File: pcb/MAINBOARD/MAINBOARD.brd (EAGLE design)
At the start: 85 x 56 mm, 67 parts, among them Q1 20MHz, SW1 P-DT6E, SW2 P-DT6E, T1 IRMLM0060TRPbF

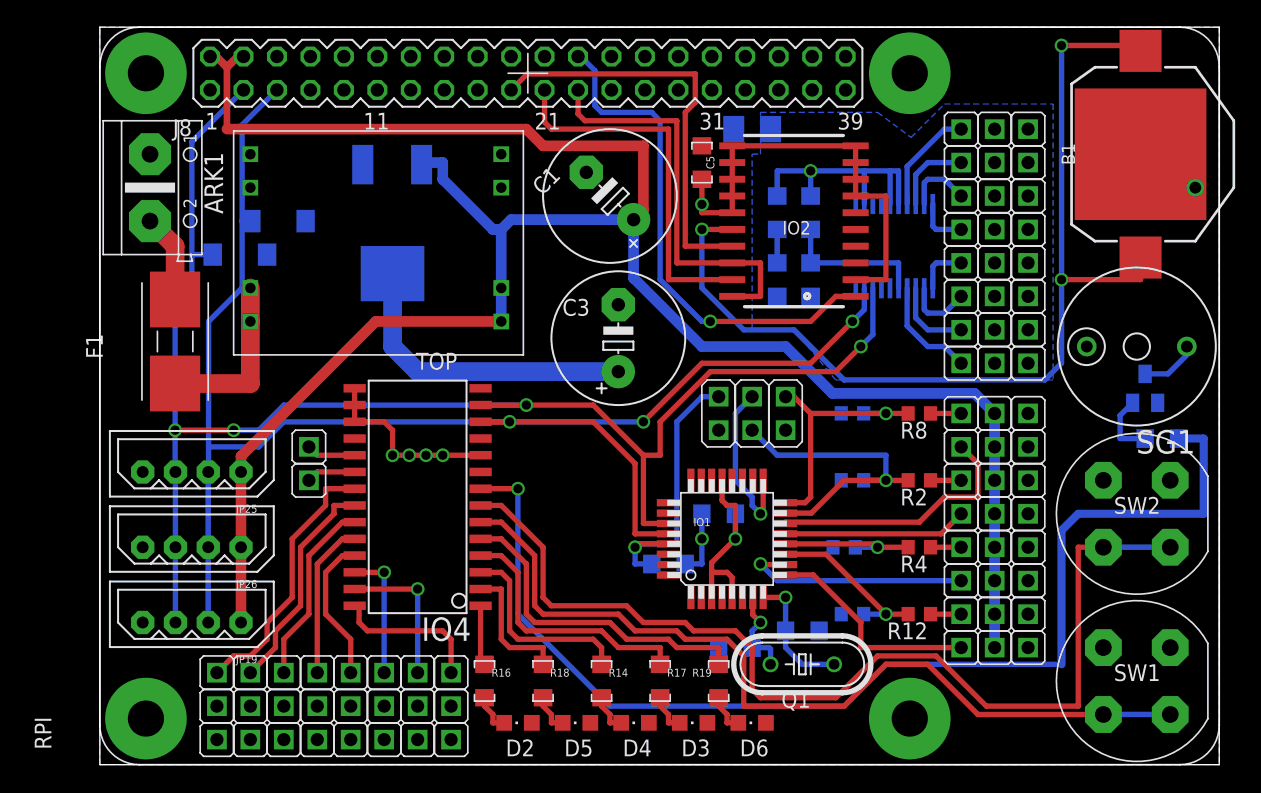
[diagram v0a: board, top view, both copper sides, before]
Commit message: Přidány opravy chyb, které se vyskytly během oživování
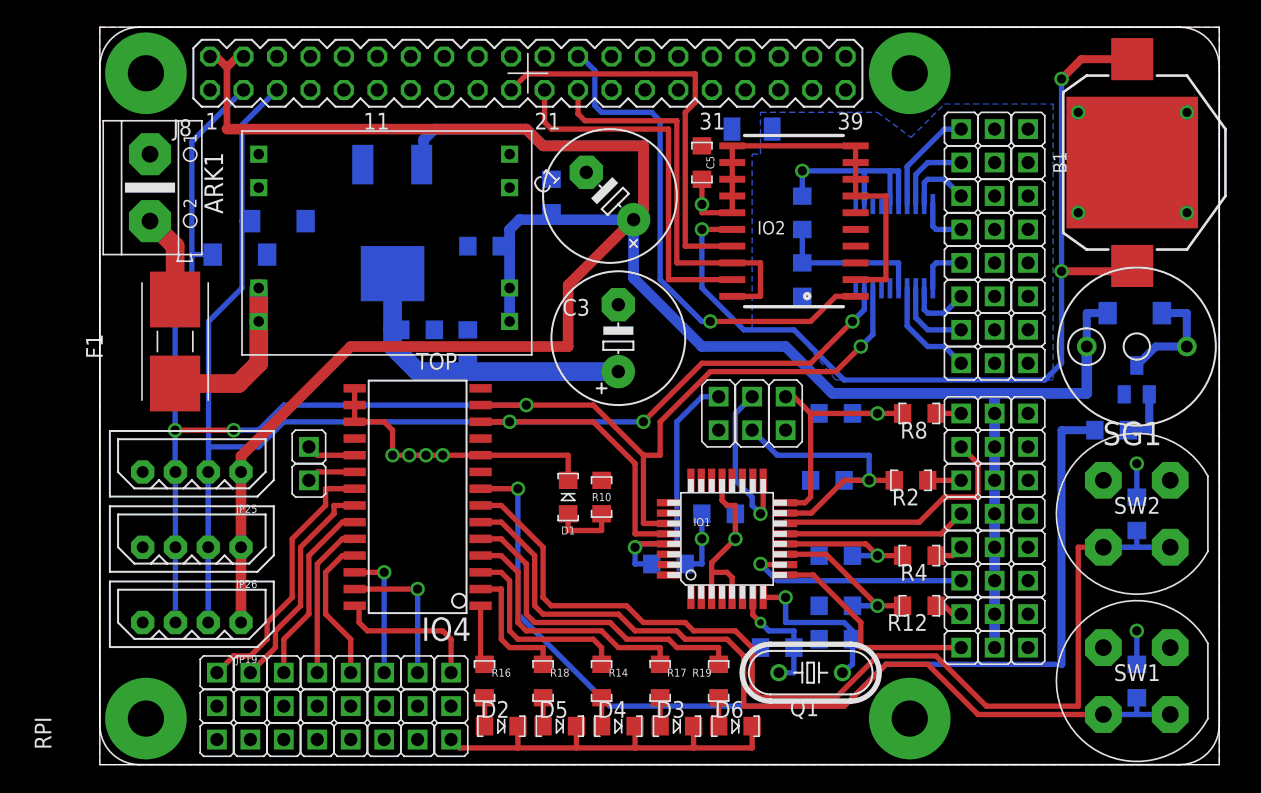
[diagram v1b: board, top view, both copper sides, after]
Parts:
- added C10, C7: 100n, !discrete:0805
- added C8, C9: 1n, !discrete:0805
- added D7: 1N4148, #PaJa_30:SOD-80
- added R20, R21: 100k, !discrete:0805
- C1, C3: value 100uF/16V -> 100uF
- D2, D3, D4, D5, D6: device led:CHIPLED_0805 -> !opto:LED_0805
- DC1: value DC-DC-STEPDOWN -> MP1584
- DZ1: value D -ZENEROVA 3.3V -> BZV55C3.3
- DZ2: value D-ZENEROVA 3.3V -> BZV55C3.3
- R1, R11, R12, R2, R3, R4, R7, R8: device rcl:R0603 -> !discrete:0805
- R10, R14, R16, R17, R18, R19: value 68R -> 330R
- R5: device rcl:M1206 -> !discrete:1206
- R6, R9: value DNP -> 10k
- T1: device transistor:SOT23-EBC -> #TD:NPN-BCE
- moved R10 25.4 mm to (38.1, 20.3), flipped to the top
- moved D1 22.9 mm to (35.6, 20.3), flipped to the top, turned to 90 degrees
- moved R15 3.86 mm to (76.8, 25.4), turned to 180 degrees
- moved C4 3.18 mm to (51.4, 8.89)
- moved C6 2.62 mm to (55.9, 9.53), turned to 180 degrees
- moved R1 1.91 mm to (55.2, 21.6)
- moved R11 1.42 mm to (55.9, 12.1)
- moved D3 1.30 mm to (43.8, 2.92), turned to 0 degrees
- moved D4 1.30 mm to (39.4, 2.92), turned to 0 degrees
- moved D5 1.30 mm to (34.9, 2.92), turned to 0 degrees
- moved D6 1.30 mm to (48.3, 2.92), turned to 0 degrees
- moved D2 1.30 mm to (30.5, 2.92), turned to 0 degrees
- moved R7 1.27 mm to (55.9, 26.7)
- moved T1 0.90 mm to (78.7, 29.2)
- moved B1 0.90 mm to (78.7, 45.7)
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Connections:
- net N$2 renamed B
- removed net N$13: D3.C, R17.2
- removed net N$15: D5.C, R18.2
- removed net N$9: D2.C, R16.2
- new net C: D7.A, SG1.-, T1.C
- new net N$2: D6.A, R19.2
- new net N$7: D2.A, R16.2
- net +3V3: now also C10.2, C9.2, R20.2, R21.2; no longer D2.A, D3.A, D4.A, D5.A, D6.A, SG1.+
- net +5V: now also C7.1, C8.1, D7.K, SG1.+
- net AGND: no longer D1.K
- net GND: now also C10.1, C7.2, C8.2, C9.1, D1.K, D2.K, D3.K, D4.K, D5.K, D6.K
- net GPB5-2: now also R20.1
- net GPB6-2: now also R21.1
- net N$3: now also D3.A, R17.2; no longer SG1.-, T1.C
- net N$4: now also D4.A, R14.2; no longer D6.C, R19.2
- net N$6: now also D5.A, R18.2; no longer D4.C, R14.2
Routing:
- net GND: track 64.3 -> 119.3 mm, vias 7 -> 10
- net +5V: track 162.8 -> 211.3 mm
- net C: track 0.00 -> 8.83 mm
- net GPB7-2: track 86.9 -> 78.2 mm
- net VBATT: track 75.7 -> 70.8 mm
- net N$15: track 3.02 -> 0.00 mm
- net N$9: track 3.02 -> 0.00 mm
- net N$13: track 3.02 -> 0.00 mm
- net XTAL2: track 9.72 -> 12.5 mm
- net N$23: track 2.54 -> 5.08 mm
- net +3V3: track 49.1 -> 51.7 mm, vias 2 -> 4
- net XTAL1: track 6.91 -> 9.27 mm
- net N$3: track 4.41 -> 2.16 mm
- net N$7: track 0.00 -> 2.16 mm
- net N$2: track 0.00 -> 2.16 mm
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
